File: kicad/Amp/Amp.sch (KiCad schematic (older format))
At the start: 31 parts, among them J1 Conn, J2 Conn, J3 Conn, J4 Conn, J5 Conn, U1 TS5A3166DBVR, U2 MCP1700

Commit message: изменено:      kicad/Amp/Amp-cache.lib 	изменено:      kicad/Amp/Amp.sch 	изменено:      kicad/Amp/Amp.sch-bak
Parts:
- D1: symbol Amp-rescue:MAX4477-My_Library-Amp-rescue-Amp-rescue-Amp-rescue -> Amp-rescue:MAX4477-My_Library-Amp-rescue-Amp-rescue-Amp-rescue-Amp-rescue
- D2: symbol Amp-rescue:TLV3501-2-My_Library-Amp-rescue-Amp-rescue-Amp-rescue -> Amp-rescue:TLV3501-2-My_Library-Amp-rescue-Amp-rescue-Amp-rescue-Amp-rescue
- J1, J2, J3, J4, J5: symbol Amp-rescue:Conn-My_Library-Amp-rescue-Amp-rescue-Amp-rescue-Amp-rescue-Amp-rescue-Amp-rescue-Amp-rescue -> Amp-rescue:Conn-My_Library-Amp-rescue-Amp-rescue-Amp-rescue-Amp-rescue-Amp-rescue-Amp-rescue-Amp-rescue-Amp-rescue
- R5: value 100k -> 200k
- Z1: symbol Amp-rescue:MCUSD18A40B12RS-My_Library-Amp-rescue-Amp-rescue-Amp-rescue -> Amp-rescue:MCUSD18A40B12RS-My_Library-Amp-rescue-Amp-rescue-Amp-rescue-Amp-rescue
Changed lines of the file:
@@
 $EndComp
 $Comp
-L Amp-rescue:Conn-My_Library-Amp-rescue-Amp-rescue-Amp-rescue-Amp-rescue-Amp-rescue-Amp-rescue-Amp-rescue J3
+L Amp-rescue:Conn-My_Library-Amp-rescue-Amp-rescue-Amp-rescue-Amp-rescue-Amp-rescue-Amp-rescue-Amp-rescue-Amp-rescue J3
 U 1 1 63C80349
 P 8600 4650
@@
 P 5400 3450
 F 0 "R5" V 5193 3450 50  0000 C CNN
-F 1 "100k" V 5284 3450 50  0000 C CNN
+F 1 "200k" V 5284 3450 50  0000 C CNN
 F 2 "Resistor_SMD:R_0402_1005Metric" V 5330 3450 50  0001 C CNN
 F 3 "~" H 5400 3450 50  0001 C CNN
@@
 $EndComp
 $Comp
-L Amp-rescue:Conn-My_Library-Amp-rescue-Amp-rescue-Amp-rescue-Amp-rescue-Amp-rescue-Amp-rescue-Amp-rescue J5
+L Amp-rescue:Conn-My_Library-Amp-rescue-Amp-rescue-Amp-rescue-Amp-rescue-Amp-rescue-Amp-rescue-Amp-rescue-Amp-rescue J5
 U 1 1 63C8F41C
 P 9150 3000
@@
 $EndComp
 $Comp
-L Amp-rescue:Conn-My_Library-Amp-rescue-Amp-rescue-Amp-rescue-Amp-rescue-Amp-rescue-Amp-rescue-Amp-rescue J4
+L Amp-rescue:Conn-My_Library-Amp-rescue-Amp-rescue-Amp-rescue-Amp-rescue-Amp-rescue-Amp-rescue-Amp-rescue-Amp-rescue J4
 U 1 1 63C92E60
 P 8600 4900
@@
 In
 $Comp
-L Amp-rescue:Conn-My_Library-Amp-rescue-Amp-rescue-Amp-rescue-Amp-rescue-Amp-rescue-Amp-rescue-Amp-rescue J1
+L Amp-rescue:Conn-My_Library-Amp-rescue-Amp-rescue-Amp-rescue-Amp-rescue-Amp-rescue-Amp-rescue-Amp-rescue-Amp-rescue J1
 U 1 1 63D437C1
 P 2950 3600
@@
 Connection ~ 8750 3000
 $Comp
-L Amp-rescue:MAX4477-My_Library-Amp-rescue-Amp-rescue-Amp-rescue D1
+L Amp-rescue:MAX4477-My_Library-Amp-rescue-Amp-rescue-Amp-rescue-Amp-rescue D1
 U 1 1 63E14065
 P 5250 3750
@@
 $EndComp
 $Comp
-L Amp-rescue:MAX4477-My_Library-Amp-rescue-Amp-rescue-Amp-rescue D1
+L Amp-rescue:MAX4477-My_Library-Amp-rescue-Amp-rescue-Amp-rescue-Amp-rescue D1
 U 2 1 63E14B3D
 P 6600 3900
@@
 $EndComp
 $Comp
-L Amp-rescue:TLV3501-2-My_Library-Amp-rescue-Amp-rescue-Amp-rescue D2
+L Amp-rescue:TLV3501-2-My_Library-Amp-rescue-Amp-rescue-Amp-rescue-Amp-rescue D2
 U 1 1 63E15A52
 P 8050 4000
@@
 	3050 3600 3150 3600
 $Comp
-L Amp-rescue:Conn-My_Library-Amp-rescue-Amp-rescue-Amp-rescue-Amp-rescue-Amp-rescue-Amp-rescue-Amp-rescue J2
+L Amp-rescue:Conn-My_Library-Amp-rescue-Amp-rescue-Amp-rescue-Amp-rescue-Amp-rescue-Amp-rescue-Amp-rescue-Amp-rescue J2
 U 1 1 63C8F7BE
 P 8600 4000
@@
 Out
 $Comp
-L Amp-rescue:MCUSD18A40B12RS-My_Library-Amp-rescue-Amp-rescue-Amp-rescue Z1
+L Amp-rescue:MCUSD18A40B12RS-My_Library-Amp-rescue-Amp-rescue-Amp-rescue-Amp-rescue Z1
 U 1 1 640B9EB9
 P 4150 4200

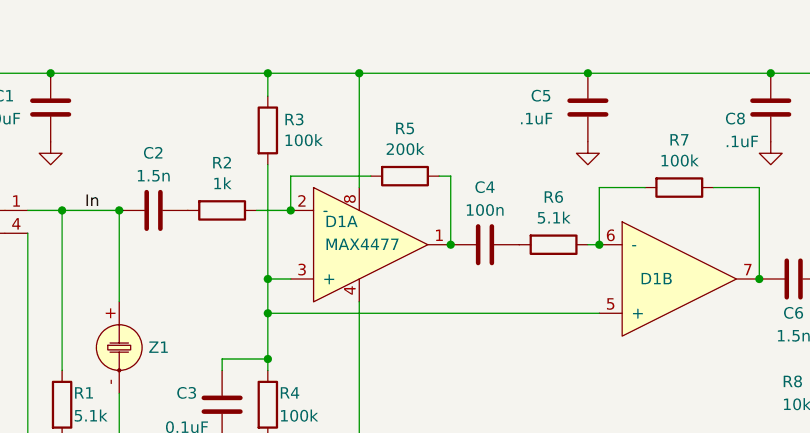
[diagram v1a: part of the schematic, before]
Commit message: изменено:      kicad/Amp/Amp.kicad_pcb 	изменено:      kicad/Amp/Amp.kicad_pcb-bak 	изменено:      kicad/Amp/Amp.sch 	изменено:      kicad/Amp/Amp.sch-bak 	изменено:      stm32cubeide/Anemometr_v3/.mxproject 	изменено:      stm32cubeide/Anemometr_v3/Anemometr_3.ioc 	изменено:      stm32cubeide/Anemometr_v3/Core/Inc/main.h 	изменено:      stm32cubeide/Anemometr_v3/Core/Inc/stm32f1xx_hal_conf.h 	изменено:      stm32cubeide/Anemometr_v3/Core/Src/main.c 	изменено:      stm32cubeide/Anemometr_v3/Core/Src/stm32f1xx_it.c 	изменено:      stm32cubeide/Anemometr_v3/Debug/Anemometr_3.bin 	изменено:      stm32cubeide/Anemometr_v3/Debug/Anemometr_3.elf 	изменено:      stm32cubeide/Anemometr_v3/Debug/Anemometr_3.list 	изменено:      stm32cubeide/Anemometr_v3/Debug/Anemometr_3.map 	изменено:      stm32cubeide/Anemometr_v3/Debug/Core/Src/BME280.d 	изменено:      stm32cubeide/Anemometr_v3/Debug/Core/Src/BME280.o 	изменено:      stm32cubeide/Anemometr_v3/Debug/Core/Src/main.d 	изменено:      stm32cubeide/Anemometr_v3/Debug/Core/Src/main.o 	изменено:      stm32cubeide/Anemometr_v3/Debug/Core/Src/main.su 	изменено:      stm32cubeide/Anemometr_v3/Debug/Core/Src/stm32f1xx_hal_msp.d 	изменено:      stm32cubeide/Anemometr_v3/Debug/Core/Src/stm32f1xx_hal_msp.o 	изменено:      stm32cubeide/Anemometr_v3/Debug/Core/Src/stm32f1xx_it.d 	изменено:      stm32cubeide/Anemometr_v3/Debug/Core/Src/stm32f1xx_it.o 	изменено:      stm32cubeide/Anemometr_v3/Debug/Core/Src/stm32f1xx_it.su 	изменено:      stm32cubeide/Anemometr_v3/Debug/Core/Src/system_stm32f1xx.d 	изменено:      stm32cubeide/Anemometr_v3/Debug/Core/Src/system_stm32f1xx.o 	изменено:      stm32cubeide/Anemometr_v3/Debug/Drivers/STM32F1xx_HAL_Driver/Src/stm32f1xx_hal.d 	изменено:      stm32cubeide/Anemometr_v3/Debug/Drivers/STM32F1xx_HAL_Driver/Src/stm32f1xx_hal.o 	изменено:      stm32cubeide/Anemometr_v3/Debug/Drivers/STM32F1xx_HAL_Driver/Src/stm32f1xx_hal_cortex.d 	изменено:      stm32cubeide/Anemometr_v3/Debug/Drivers/STM32F1xx_HAL_Driver/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
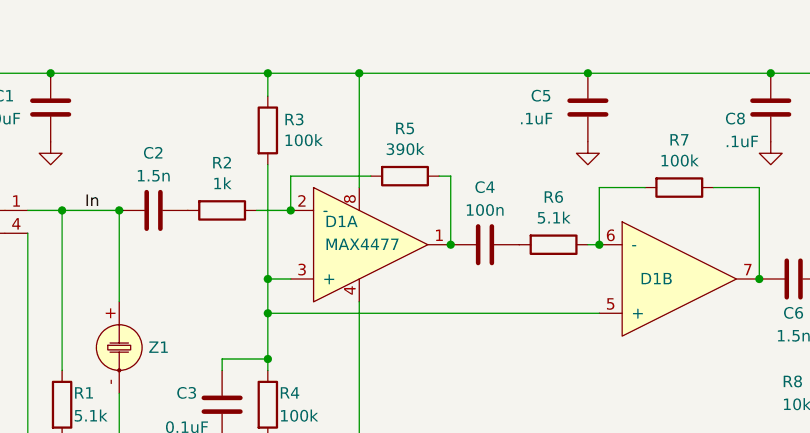
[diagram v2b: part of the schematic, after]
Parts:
- R5: value 200k -> 390k
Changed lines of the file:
@@
 P 5400 3450
 F 0 "R5" V 5193 3450 50  0000 C CNN
-F 1 "200k" V 5284 3450 50  0000 C CNN
+F 1 "390k" V 5284 3450 50  0000 C CNN
 F 2 "Resistor_SMD:R_0402_1005Metric" V 5330 3450 50  0001 C CNN
 F 3 "~" H 5400 3450 50  0001 C CNN

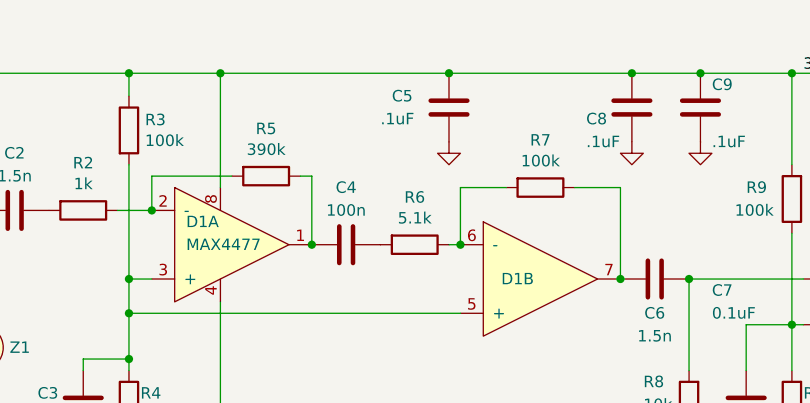
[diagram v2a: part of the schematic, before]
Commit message: изменено:      kicad/Amp/Amp.kicad_pcb 	изменено:      kicad/Amp/Amp.kicad_pcb-bak 	изменено:      kicad/Amp/Amp.sch 	изменено:      kicad/Amp/Amp.sch-bak 	изменено:      kicad/Amp/fp-info-cache
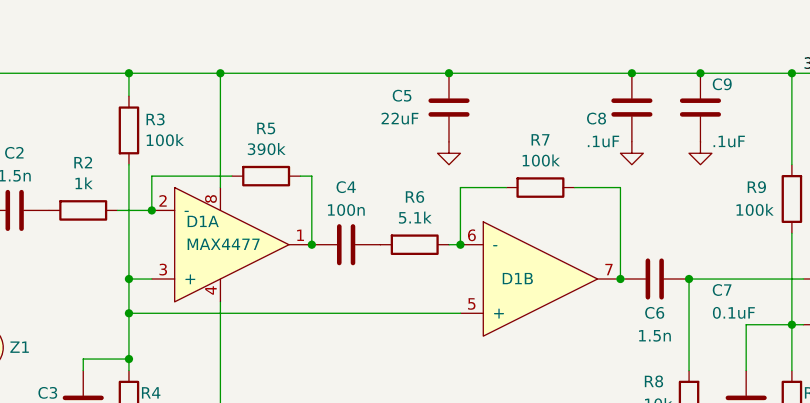
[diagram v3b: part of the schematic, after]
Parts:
- C5: value .1uF -> 22uF; footprint Capacitor_SMD:C_0603_1608Metric -> Capacitor_SMD:C_0805_2012Metric
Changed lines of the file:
@@
 P 6200 3150
 F 0 "C5" H 5950 3200 50  0000 L CNN
-F 1 ".1uF" H 5900 3100 50  0000 L CNN
-F 2 "Capacitor_SMD:C_0603_1608Metric" H 6238 3000 50  0001 C CNN
+F 1 "22uF" H 5900 3100 50  0000 L CNN
+F 2 "Capacitor_SMD:C_0805_2012Metric" H 6238 3000 50  0001 C CNN
 F 3 "~" H 6200 3150 50  0001 C CNN
 	1    6200 3150

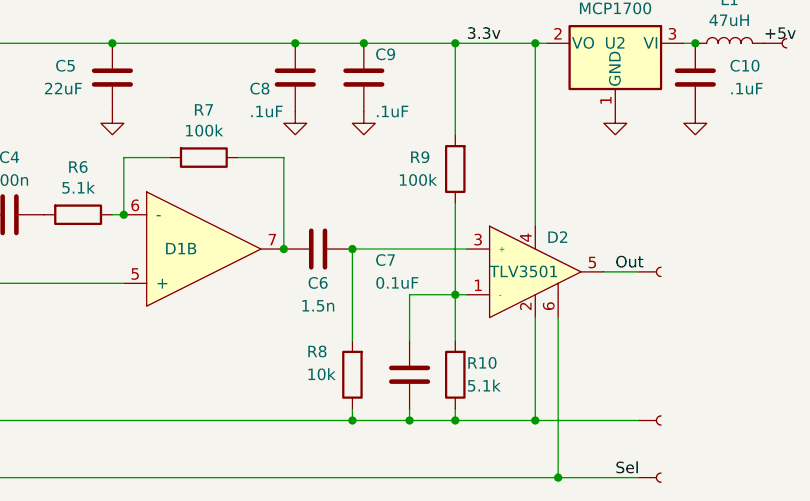
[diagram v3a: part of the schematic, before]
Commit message: изменено:      kicad/Amp/Amp.kicad_pcb 	изменено:      kicad/Amp/Amp.kicad_pcb-bak 	изменено:      kicad/Amp/Amp.sch 	изменено:      kicad/Amp/Amp.sch-bak 	изменено:      stm32cubeide/Anemometr_v3/Core/Inc/main.h 	изменено:      stm32cubeide/Anemometr_v3/Core/Src/stm32f1xx_it.c 	изменено:      stm32cubeide/Anemometr_v3/Debug/Anemometr_3.bin 	изменено:      stm32cubeide/Anemometr_v3/Debug/Anemometr_3.elf 	изменено:      stm32cubeide/Anemometr_v3/Debug/Anemometr_3.list 	изменено:      stm32cubeide/Anemometr_v3/Debug/Anemometr_3.map 	изменено:      stm32cubeide/Anemometr_v3/Debug/Core/Src/BME280.o 	изменено:      stm32cubeide/Anemometr_v3/Debug/Core/Src/main.o 	изменено:      stm32cubeide/Anemometr_v3/Debug/Core/Src/main.su 	изменено:      stm32cubeide/Anemometr_v3/Debug/Core/Src/stm32f1xx_hal_msp.o 	изменено:      stm32cubeide/Anemometr_v3/Debug/Core/Src/stm32f1xx_it.o
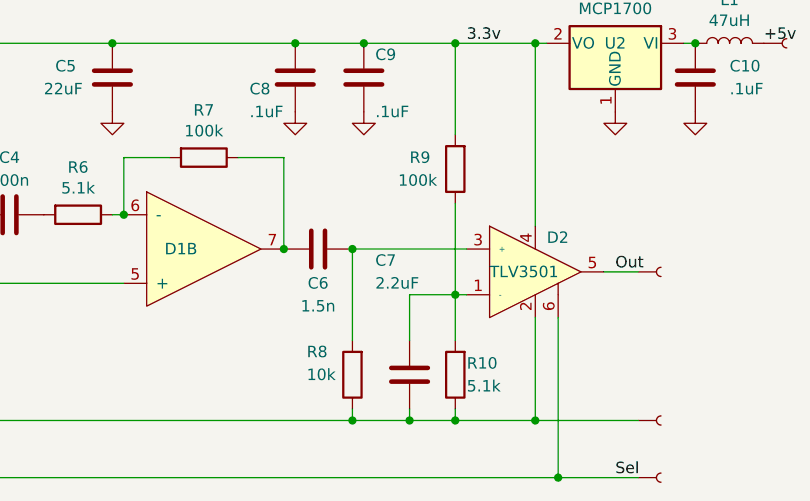
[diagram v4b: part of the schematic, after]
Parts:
- C7: value 0.1uF -> 2.2uF
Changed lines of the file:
@@
 P 7500 4450
 F 0 "C7" H 7350 4950 50  0000 L CNN
-F 1 "0.1uF" H 7350 4850 50  0000 L CNN
+F 1 "2.2uF" H 7350 4850 50  0000 L CNN
 F 2 "Capacitor_SMD:C_0402_1005Metric" H 7538 4300 50  0001 C CNN
 F 3 "~" H 7500 4450 50  0001 C CNN
